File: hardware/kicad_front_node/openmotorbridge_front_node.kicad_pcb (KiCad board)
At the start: 4 copper layers, 82 x 50 mm, 49 parts, among them J1 JST_GH_04P_BACKBONE, J10 JST_PH_02P_NAVI_PWR, J4 JST_GH_06P_HUB_EXT, J7 USB_C_SERVICE, J8 JST_PH_02P_CAM_PWR, K1 CPC1017N_CAN_RELAY, Q1 DMN63D8_BSD_MOSFET, Q2 TPS1H100_AUX_LIGHT, SW1 BOOT, SW2 RESET, U1 ESP32-P4-NR16, U2 USB2514Bi-AEZG, U3 TPS54302_5V_BUCK, U4 TPS2051B_PORT2_GATE, U5 SW3526_USB_PD1_30W, U6 TCAN334G_CAN, U7 TLV75533P_3V3_LDO, U9 ESP32-E22-WROOM-2X2, Y1 24.000MHz

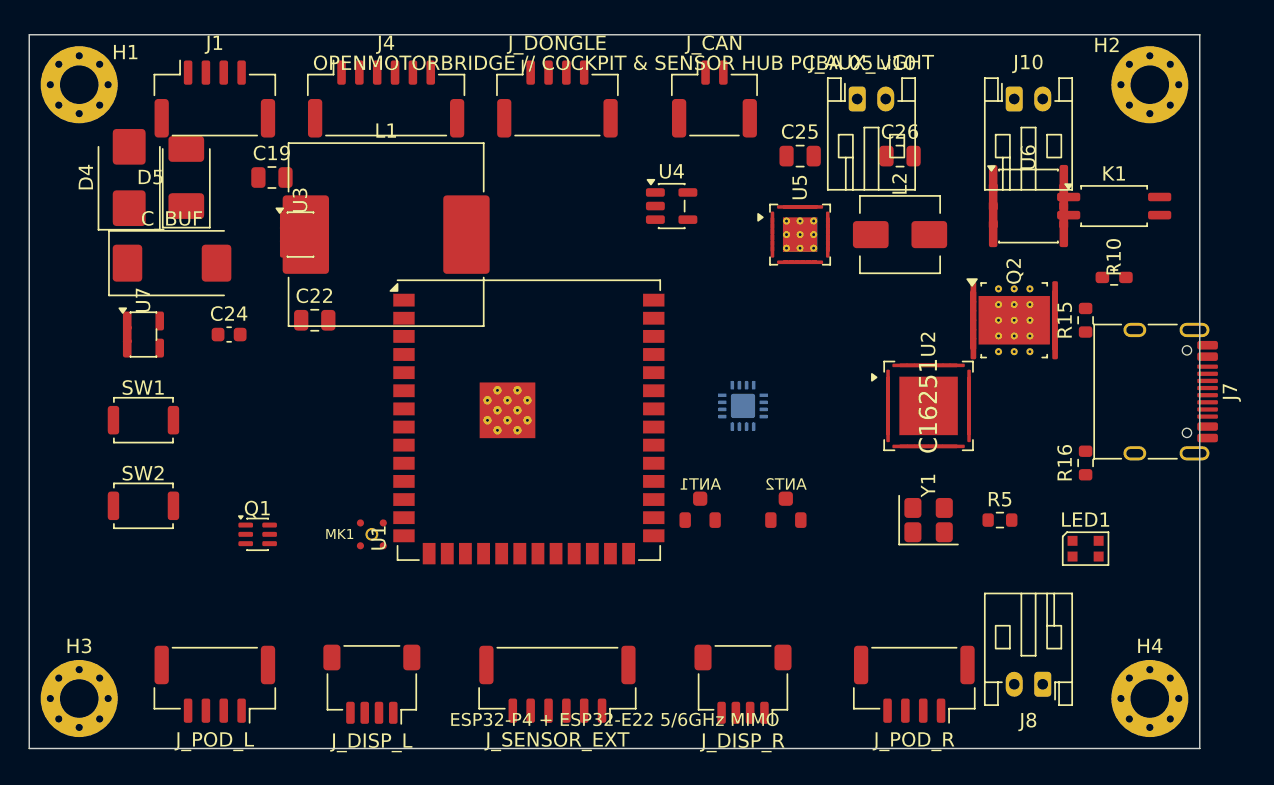
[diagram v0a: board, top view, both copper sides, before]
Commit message: hardware(front-node): connect all nets in schematic and PCB with passives parity
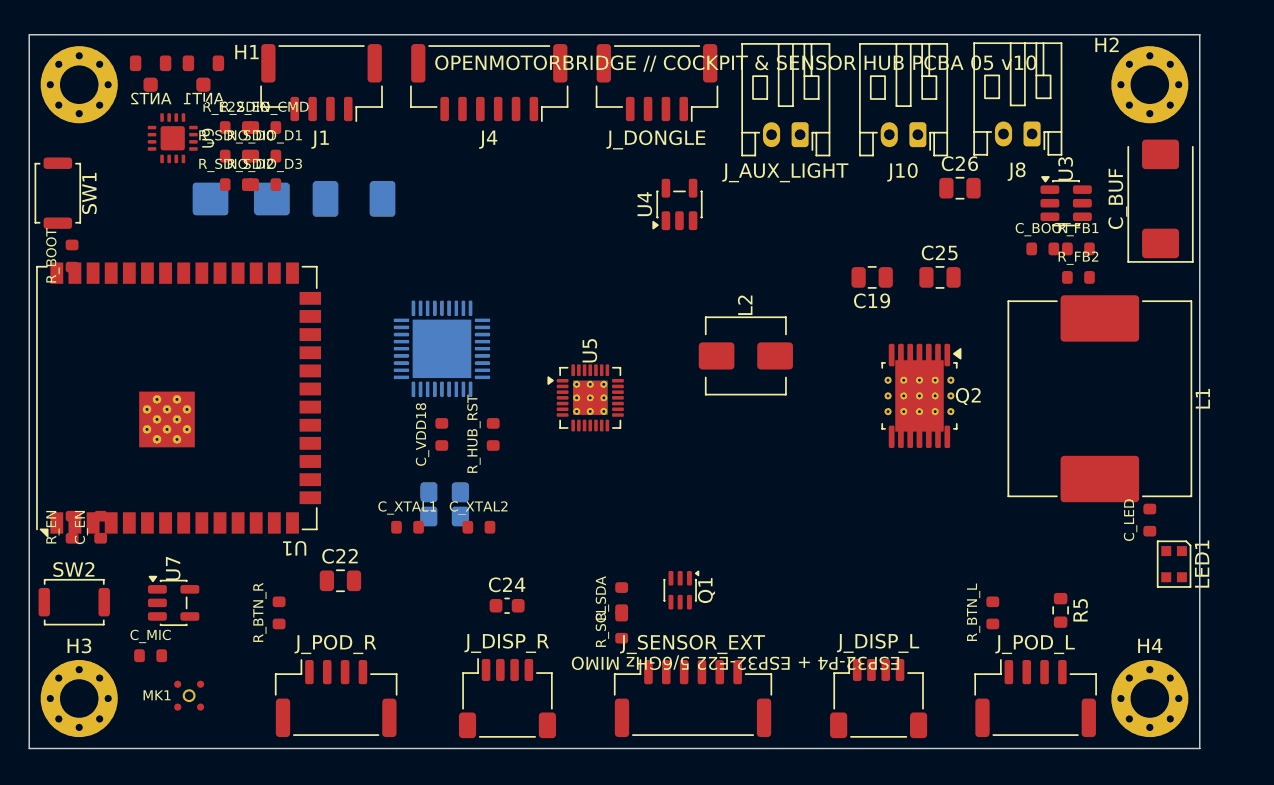
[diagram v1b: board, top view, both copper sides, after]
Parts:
- removed J7: USB_C_SERVICE, USB_C_Receptacle_HRO_TYPE-C-31-M-12
- removed J_CAN: JST_GH_02P_CAN, JST_GH_SM02B-GHS-TB_1x02-1MP_P1.25mm_Horizontal
- removed K1: CPC1017N_CAN_RELAY, SOP-4_4.4x2.6mm_P1.27mm
- removed R10: 120R_CAN, R_0603_1608Metric
- removed R15: 5.1k_CC1, R_0603_1608Metric
- removed R16: 5.1k_CC2, R_0603_1608Metric
- removed U6: TCAN334G_CAN, SOIC-8_3.9x4.9mm_P1.27mm
- added C_BOOT: 100nF, Capacitor_SMD:C_0603_1608Metric, F.Cu at (171.0, 85.0)
- added C_EN: 1uF, Capacitor_SMD:C_0603_1608Metric, F.Cu at (105.0, 104.5)
- added C_LED: 100nF, Capacitor_SMD:C_0603_1608Metric, F.Cu at (178.5, 104.0)
- added C_MIC: 100nF, Capacitor_SMD:C_0603_1608Metric, F.Cu at (108.5, 113.5)
- added C_VDD18: 1uF, Capacitor_SMD:C_0603_1608Metric, F.Cu at (128.9, 98.0)
- added C_XTAL1: 18pF, Capacitor_SMD:C_0603_1608Metric, F.Cu at (126.5, 104.5)
- added C_XTAL2: 18pF, Capacitor_SMD:C_0603_1608Metric, F.Cu at (131.5, 104.5)
- added R_BOOT: 10k, Resistor_SMD:R_0603_1608Metric, F.Cu at (103.0, 85.5)
- added R_BTN_L: 10k, Resistor_SMD:R_0603_1608Metric, F.Cu at (167.5, 110.5)
- added R_BTN_R: 10k, Resistor_SMD:R_0603_1608Metric, F.Cu at (117.5, 110.5)
- added R_E22_EN: 10k, Resistor_SMD:R_0603_1608Metric, F.Cu at (114.5, 76.5)
- added R_EN: 10k, Resistor_SMD:R_0603_1608Metric, F.Cu at (103.0, 104.5)
- added R_FB1: 100k, Resistor_SMD:R_0603_1608Metric, F.Cu at (173.5, 85.0)
- added R_FB2: 13.7k, Resistor_SMD:R_0603_1608Metric, F.Cu at (173.5, 87.0)
- added R_HUB_RST: 10k, Resistor_SMD:R_0603_1608Metric, F.Cu at (132.5, 98.0)
- added R_SCL: 4.7k, Resistor_SMD:R_0603_1608Metric, F.Cu at (141.5, 111.5)
- added R_SDA: 4.7k, Resistor_SMD:R_0603_1608Metric, F.Cu at (141.5, 109.5)
- added R_SDIO_CMD: 10k, Resistor_SMD:R_0603_1608Metric, F.Cu at (116.5, 76.5)
- added R_SDIO_D0: 10k, Resistor_SMD:R_0603_1608Metric, F.Cu at (114.5, 78.5)
- added R_SDIO_D1: 10k, Resistor_SMD:R_0603_1608Metric, F.Cu at (116.5, 78.5)
- added R_SDIO_D2: 10k, Resistor_SMD:R_0603_1608Metric, F.Cu at (114.5, 80.5)
- added R_SDIO_D3: 10k, Resistor_SMD:R_0603_1608Metric, F.Cu at (116.5, 80.5)
- D4, D5, U2, Y1: moved to B.Cu
- U9: moved to F.Cu
- moved C_BUF 69.4 mm to (179.2, 81.5), turned to 90 degrees
- moved J_POD_L 57.5 mm to (170.5, 116.5), turned to 0 degrees
- moved ANT2 54.8 mm to (108.5, 72.0), turned to 180 degrees
- moved U3 53.7 mm to (172.6, 81.8)
- moved L1 51.3 mm to (175.0, 95.5), turned to -90 degrees
- moved ANT1 47.3 mm to (112.2, 72.0), turned to 180 degrees
- moved U9 44.1 mm to (110.0, 77.2), turned to 90 degrees
- moved C19 42.6 mm to (159.1, 87.0), turned to 180 degrees
- moved J_POD_R 40.5 mm to (121.5, 116.5), turned to 0 degrees
- moved J8 38.6 mm to (170.2, 77.0)
- moved J_DISP_L 35.5 mm to (159.5, 116.5), turned to 0 degrees
- moved U2 34.3 mm to (128.9, 92.0), turned to 90 degrees
- moved Y1 33.9 mm to (129.1, 102.9), turned to 180 degrees
- moved Q1 29.9 mm to (145.6, 108.9), turned to -90 degrees
- moved C24 27.2 mm to (133.5, 110.0)
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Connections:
- ANT1 pad 1: UWB_RF -> E22_RF_MAIN
- ANT2 pad 1: UWB_RF -> E22_RF_MIMO
- C_BUF pad 1: VCC_5V -> +12V_PROT
- D4 pad 1: +12V_PROT -> VIN_60W
- D5 pad 1: KL15_12V_SW -> VIN_60W
- L1 pad 2: VBUS_BUCK_OUT -> VCC_5V
- LED1 pad 1: VCC_5V -> (no net)
- LED1 pad 2: GND -> WS2812B_DIN
- LED1 pad 3: GND -> VCC_5V
- LED1 pad 4: WS2812B_DIN -> GND
- MK1 pad 4: VCC_3V3 -> GND
- Q1 pad 3: BSD_RIGHT_N -> BSD_LED_R_N
- Q1 pad 6: BSD_LEFT_N -> BSD_LED_L_N
- Q2 pad 11: +12V_PROT -> (no net)
- Q2 pad 12: +12V_PROT -> (no net)
- Q2 pad 13: +12V_PROT -> (no net)
- Q2 pad 14: +12V_PROT -> (no net)
- Q2 pad 15: +12V_PROT -> GND
- Q2 pad 3: VCC_3V3 -> +12V_PROT
- Q2 pad 4: GND -> +12V_AUX
- Q2 pad 6: +12V_AUX -> (no net)
- Q2 pad 7: +12V_AUX -> (no net)
- Q2 pad 8: +12V_AUX -> (no net)
- U1 pad 10: PTT_IN3_N -> (no net)
- U1 pad 13: USB_SERV_DM -> USB_HS_DM
- U1 pad 14: USB_SERV_DP -> USB_HS_DP
- U1 pad 15: CAN_TERM_EN -> (no net)
- U1 pad 23: TWAI_TX -> (no net)
- U1 pad 24: USB_SERV_DM -> (no net)
- U1 pad 25: USB_SERV_DP -> (no net)
- U1 pad 30: UWB_SCK -> SDIO_CLK
- U1 pad 31: UWB_MOSI -> SDIO_CMD
- U1 pad 32: UWB_MISO -> SDIO_D0
- U1 pad 33: UWB_CS -> SDIO_D1
- U1 pad 34: UWB_IRQ -> SDIO_D2
- U1 pad 35: UWB_RST -> SDIO_D3
- U1 pad 36: TWAI_RX -> (no net)
- U1 pad 38: OTTOCAST_FAULT_N -> CP2AA_FAULT_N
- U1 pad 39: OTTOCAST_PWR_EN -> CP2AA_PWR_EN
- U1 pad 40: GND -> E22_EN
- U1 pad 5: CAN_SILENT -> (no net)
- U1 pad 8: PTT_IN1_N -> BTN_SIG_L_N
- U1 pad 9: PTT_IN2_N -> BTN_SIG_R_N
- U2 pad 11: GND -> VCC_3V3
- U2 pad 12: VCC_3V3 -> XTAL_IN
- U2 pad 13: VCC_3V3 -> XTAL_OUT
- U2 pad 17: OTTOCAST_FAULT_N -> VCC_3V3
- U2 pad 20: VCC_3V3 -> USB_UP_DM
- U2 pad 21: VCC_3V3 -> USB_UP_DP
- U2 pad 23: VCC_3V3 -> GND
- U2 pad 24: VCC_3V3 -> VCC_5V
- U2 pad 26: VCC_3V3 -> GND
- U2 pad 27: VCC_3V3 -> GND
- U2 pad 30: USB_UP_DM -> VCC_3V3
- U2 pad 31: USB_UP_DP -> VDD18_CORE
- U2 pad 32: XTAL_OUT -> VCC_3V3
- U2 pad 33: XTAL_IN -> HUB_RESET_N
- U2 pad 35: HUB_RBIAS -> VCC_3V3
- U2 pad 36: VCC_3V3 -> HUB_RBIAS
- U2 pad 8: USB_DN4_DM -> USB_HS_DM
- U2 pad 9: USB_DN4_DP -> USB_HS_DP
- U3 pad 4: VCC_5V -> FB_5V
- U3 pad 6: SW_BUCK -> BOOT_5V
- U4 pad 1: VCC_5V_OTTOCAST -> VCC_5V
- U4 pad 3: OTTOCAST_FAULT_N -> CP2AA_PWR_EN
- U4 pad 4: OTTOCAST_PWR_EN -> CP2AA_FAULT_N
- U4 pad 5: VCC_5V -> VCC_5V_DONGLE
- U5 pad 14: GND -> (no net)
- U5 pad 16: USB_DN1_DP -> (no net)
- U5 pad 17: USB_DN1_DM -> (no net)
- U5 pad 18: USB_DN1_CC -> (no net)
- U5 pad 19: USB_DN1_CC -> (no net)
- U5 pad 2: +12V_PROT -> SW_PD1_BUCK
- U5 pad 21: VBUS_PD1_OUT -> (no net)
- U5 pad 25: SW_PD1_BUCK -> (no net)
- U5 pad 26: SW_PD1_BUCK -> (no net)
- U5 pad 27: SW_PD1_BUCK -> (no net)
- U5 pad 28: +12V_PROT -> (no net)
- U7 pad 4: GND -> (no net)
- U9 pad 1: GND -> VCC_3V3
- U9 pad 10: UWB_CS -> E22_IRQ
- U9 pad 11: GND -> E22_RF_MAIN
- U9 pad 12: UWB_RST -> E22_RF_MIMO
- U9 pad 13: UWB_IRQ -> GND
- U9 pad 14: VCC_3V3 -> GND
- U9 pad 15: UWB_RF -> GND
- U9 pad 3: GND -> E22_EN
- U9 pad 4: UWB_XTAL1 -> SDIO_CLK
- U9 pad 5: UWB_XTAL2 -> SDIO_CMD
- U9 pad 6: GND -> SDIO_D0
- U9 pad 7: UWB_SCK -> SDIO_D1
- U9 pad 8: UWB_MISO -> SDIO_D2
- U9 pad 9: UWB_MOSI -> SDIO_D3
